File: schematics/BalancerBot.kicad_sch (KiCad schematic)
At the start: 7 parts, among them M1 Motor_DC, M2 Motor_DC, U1 MCP73871, U2 L298N

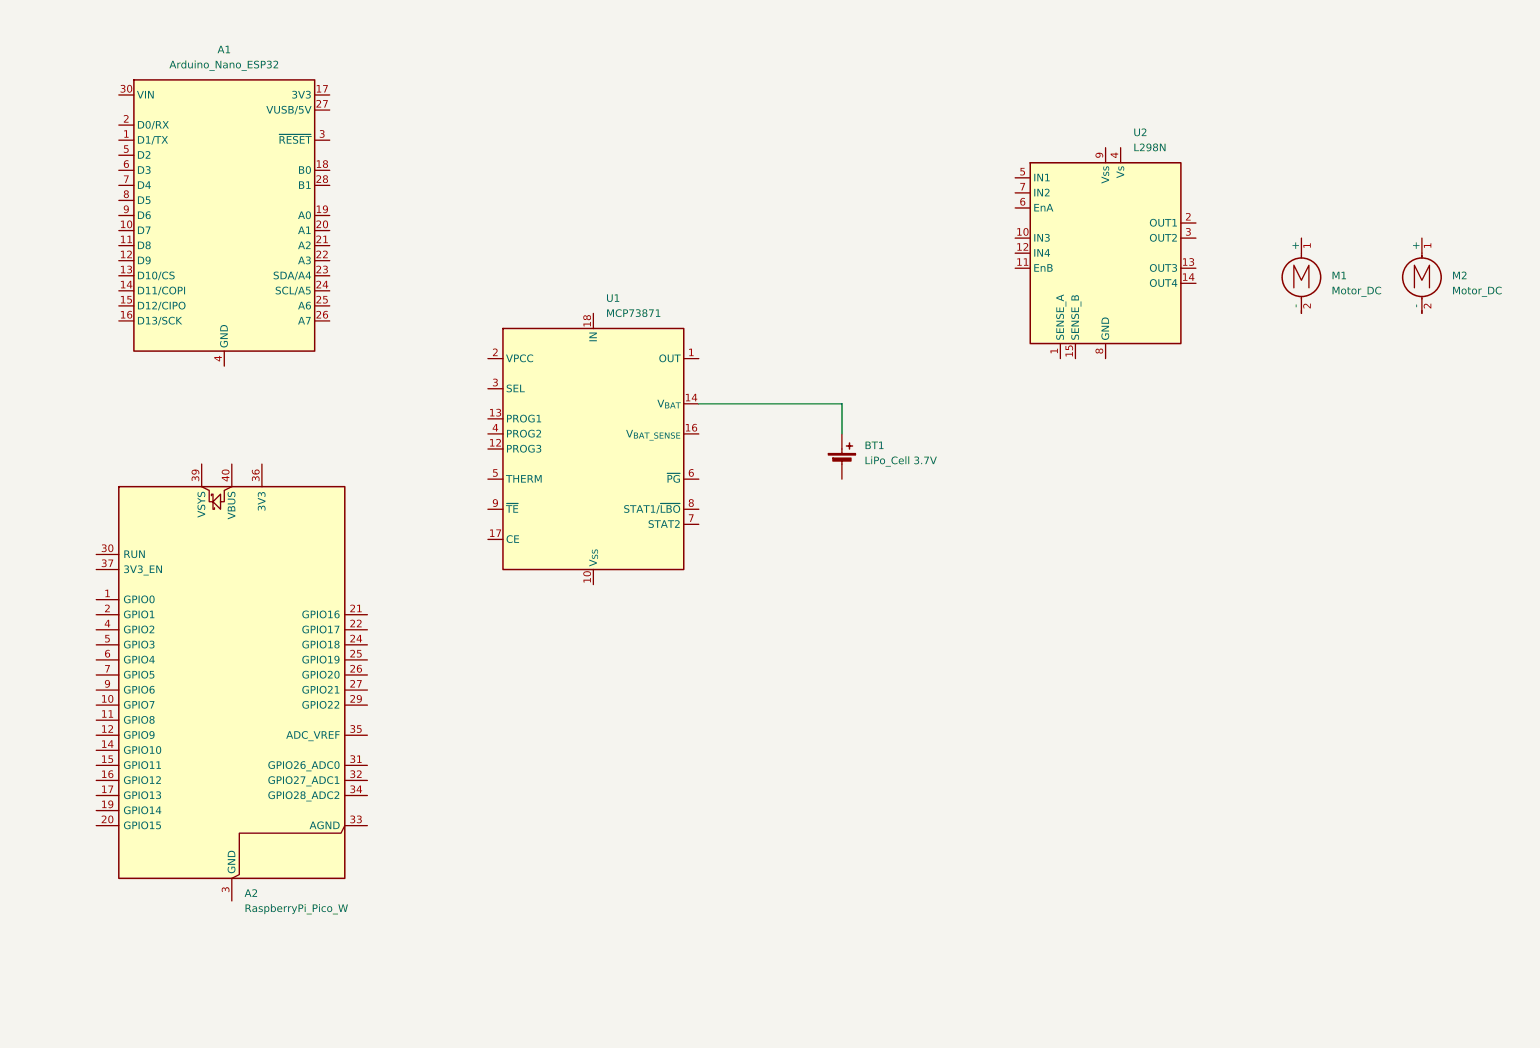
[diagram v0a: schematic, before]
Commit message: Update
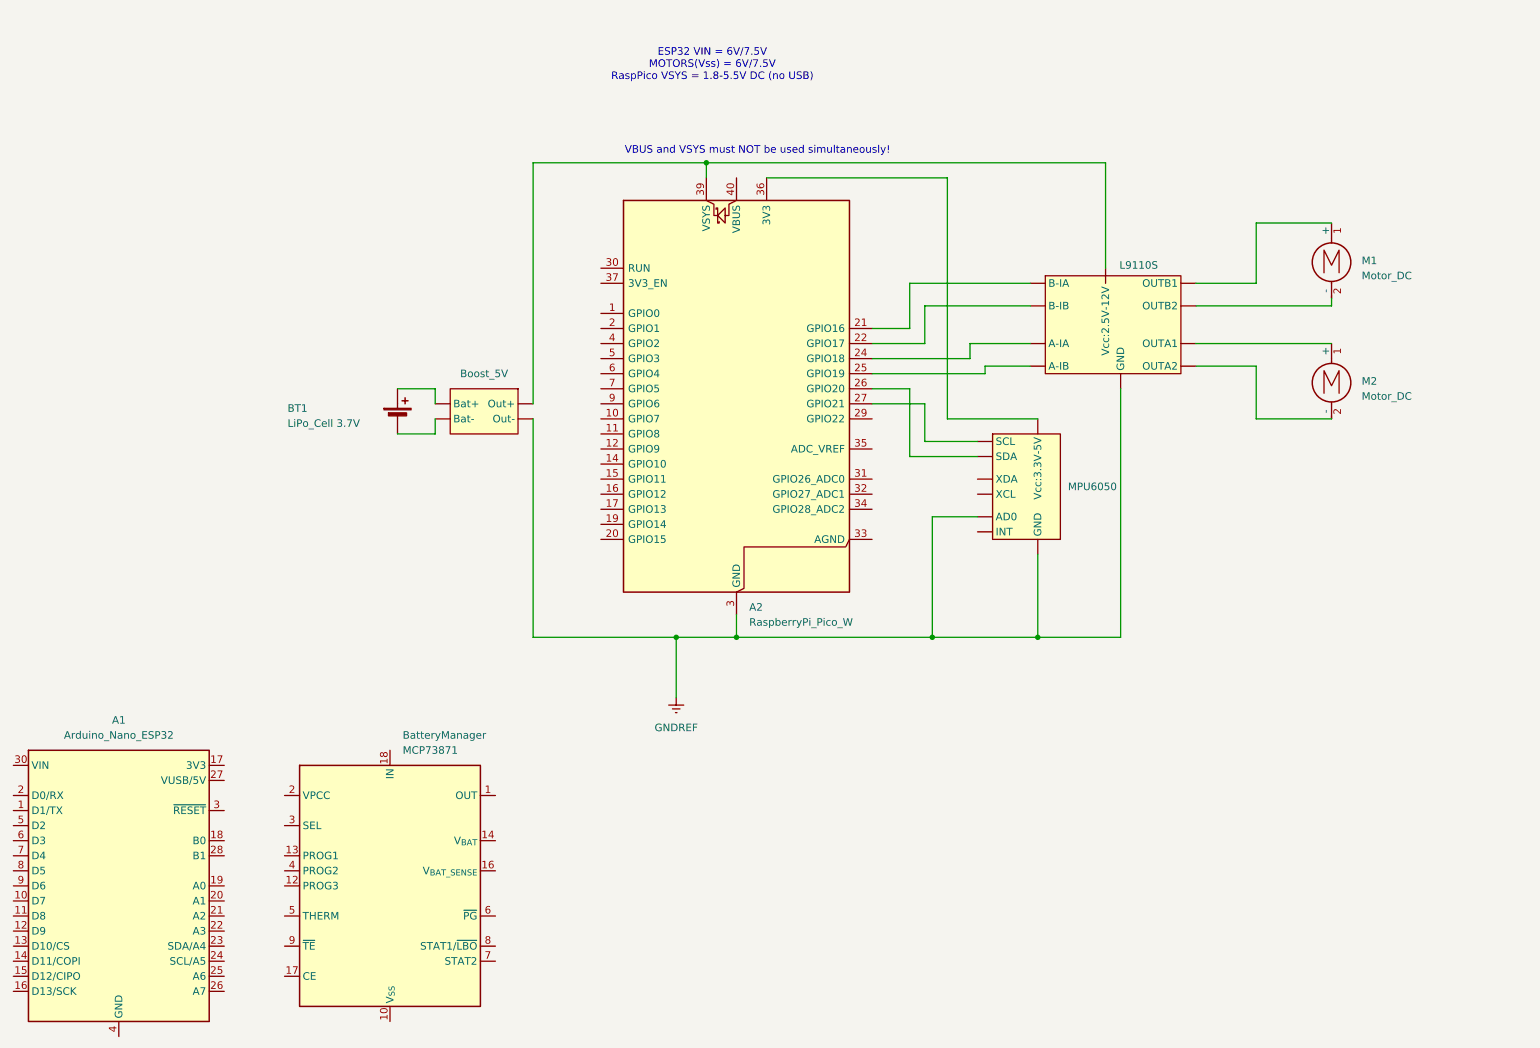
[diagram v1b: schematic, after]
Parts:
- removed U2: L298N, Package_TO_SOT_THT:TO-220-15_P2.54x5.08mm_StaggerOdd_Lead4.58mm_Vertical, symbol Driver_Motor:L298N
- added Boost_5V: (no value), symbol 1MyLibrary:Power_Boost_module_-_5V_0.5A_JST
- added L9110S: (no value), symbol MyLibrary:L9110S
- added MPU6050: (no value), symbol 1MyLibrary:SEN-MPU6050
- renumbered U1 to BatteryManager
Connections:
- net at M2.1 (+): now also L9110S. (OUTA2)
- net at M2.2 (-): now also L9110S. (OUTA2)
- net at BatteryManager.14 (V_{BAT}), BatteryManager.15 (V_{BAT}): no longer BT1.1 (+)
- net at BT1.2 (-): now also Boost_5V. (Bat-)
- net at M1.1 (+): now also L9110S. (OUTA2)
- net at M1.2 (-): now also L9110S. (OUTA2)
- net GNDREF: now reaches A2.13 (GND), A2.18 (GND), A2.23 (GND), A2.28 (GND), A2.3 (GND), A2.38 (GND), A2.8 (GND)
- net GNDREF: now also Boost_5V. (Bat-), L9110S. (OUTA2), MPU6050. (GND)
- net at A2.21 (GPIO16): now also L9110S. (OUTA2)
- net at A2.22 (GPIO17): now also L9110S. (OUTA2)
- net at A2.24 (GPIO18): now also L9110S. (OUTA2)
- net at A2.25 (GPIO19): now also L9110S. (OUTA2)
- net at A2.26 (GPIO20): now also MPU6050. (GND)
- net at A2.27 (GPIO21): now also MPU6050. (GND)
- net at A2.36 (3V3): now also MPU6050. (GND)
- net at A2.39 (VSYS): now also Boost_5V. (Bat-), L9110S. (OUTA2)
- new net: BT1.1 (+), Boost_5V. (Bat-)
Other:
- note added: "ESP32 VIN = 6V/7.5V MOTORS(Vss) = 6V/7.5V RaspPico VSYS = 1.8-5.5V DC (no USB)"
- note added: "VBUS and VSYS must NOT be used simultaneously!"
- moved on the sheet: A1, A2, BT1, BatteryManager, M1, M2

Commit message: Update schematic
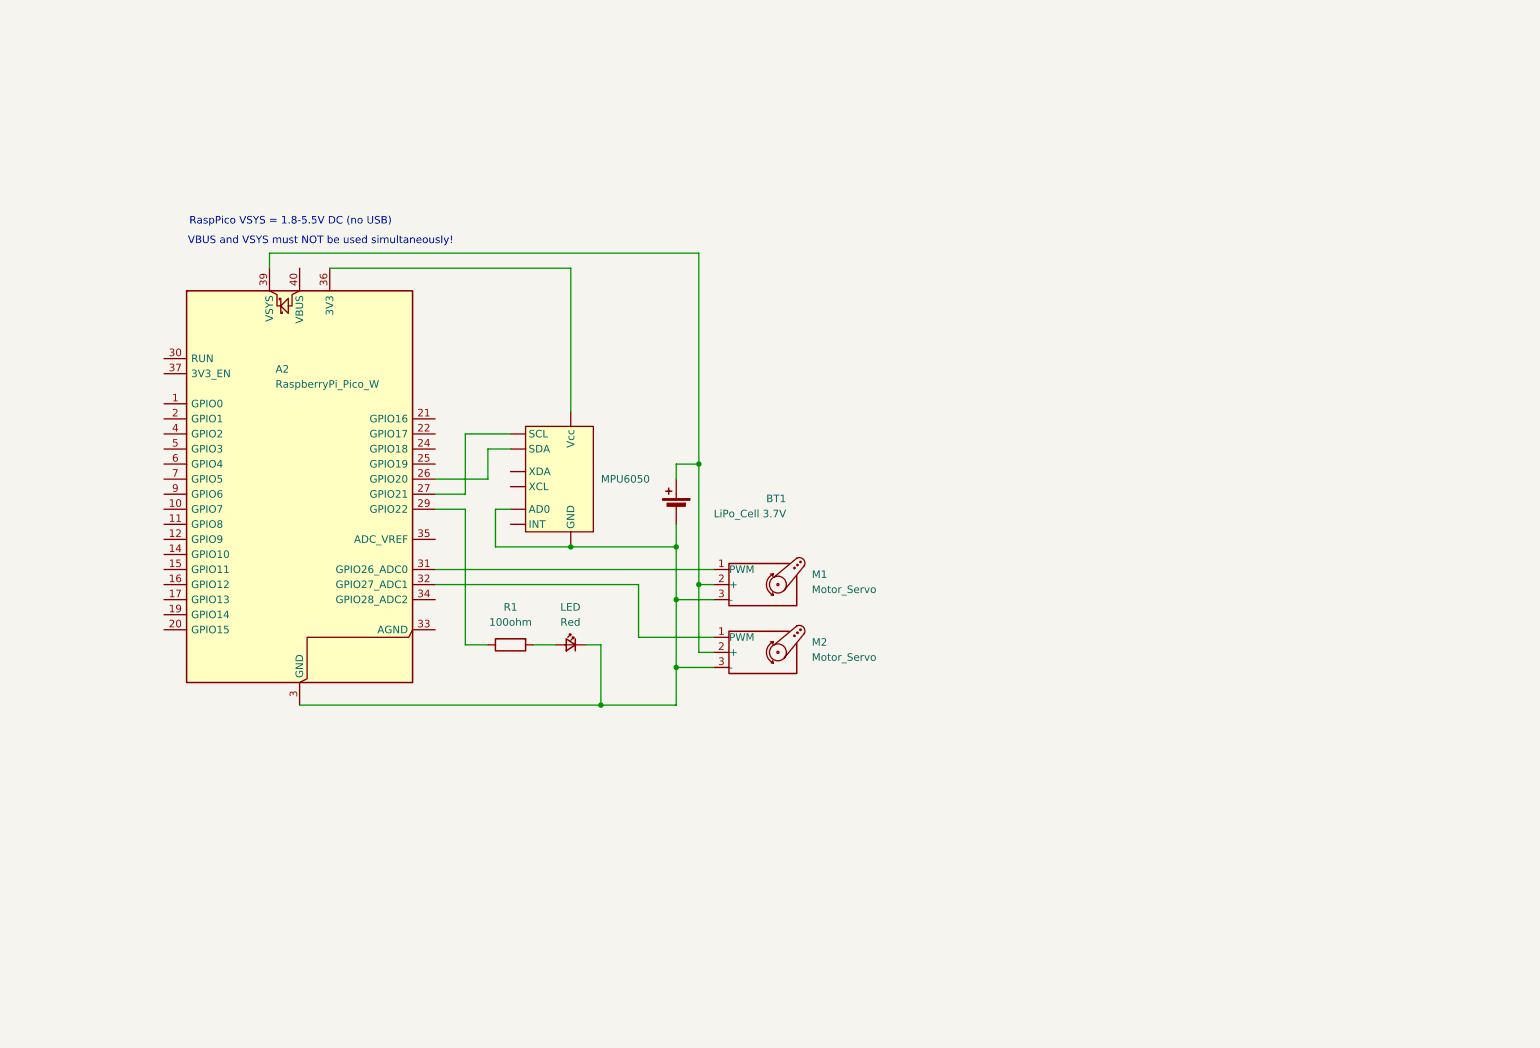
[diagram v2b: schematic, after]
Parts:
- removed A1: Arduino_Nano_ESP32, Module:Arduino_Nano, symbol MCU_Module:Arduino_Nano_ESP32
- removed BatteryManager: MCP73871, Package_DFN_QFN:QFN-20-1EP_4x4mm_P0.5mm_EP2.5x2.5mm, symbol Battery_Management:MCP73871
- removed Boost_5V: (no value), symbol 1MyLibrary:Power_Boost_module_-_5V_0.5A_JST
- removed L9110S: (no value), symbol MyLibrary:L9110S
- removed M1, M2: Motor_DC, symbol Motor:Motor_DC
- added LED: Red, PCM_SparkFun-LED:LED_0402_1005Metric_Red, symbol PCM_SparkFun-LED:LED_Red_0402
- added M1, M2: Motor_Servo, symbol Motor:Motor_Servo
- added R1: 100ohm, symbol PCM_Resistor_AKL:R_Generic
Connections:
- net at MPU6050. (GND): now also A2.36 (3V3)
- net at BT1.1 (+): now also A2.39 (VSYS), M1.2 (+), M2.2 (+)
- net at BT1.2 (-): now also A2.13 (GND), A2.18 (GND), A2.23 (GND), A2.28 (GND), A2.3 (GND), A2.38 (GND), A2.8 (GND), MPU6050. (GND), LED.1 (K), M1.3 (-), M2.3 (-)
- net at A2.29 (GPIO22): now also R1.2
- net at A2.31 (GPIO26_ADC0): now also M1.1 (PWM)
- net at A2.32 (GPIO27_ADC1): now also M2.1 (PWM)
- removed net GNDREF: A2.13 (GND), A2.18 (GND), A2.23 (GND), A2.28 (GND), A2.3 (GND), A2.38 (GND), A2.8 (GND), MPU6050. (GND)
- new net: LED.2 (A), R1.1
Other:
- note added: "RaspPico VSYS = 1.8-5.5V DC (no USB)"
- note removed: "ESP32 VIN = 6V/7.5V MOTORS(Vss) = 6V/7.5V RaspPico VSYS = 1.8-5.5V DC (no USB)"
- moved on the sheet: A2, BT1, MPU6050

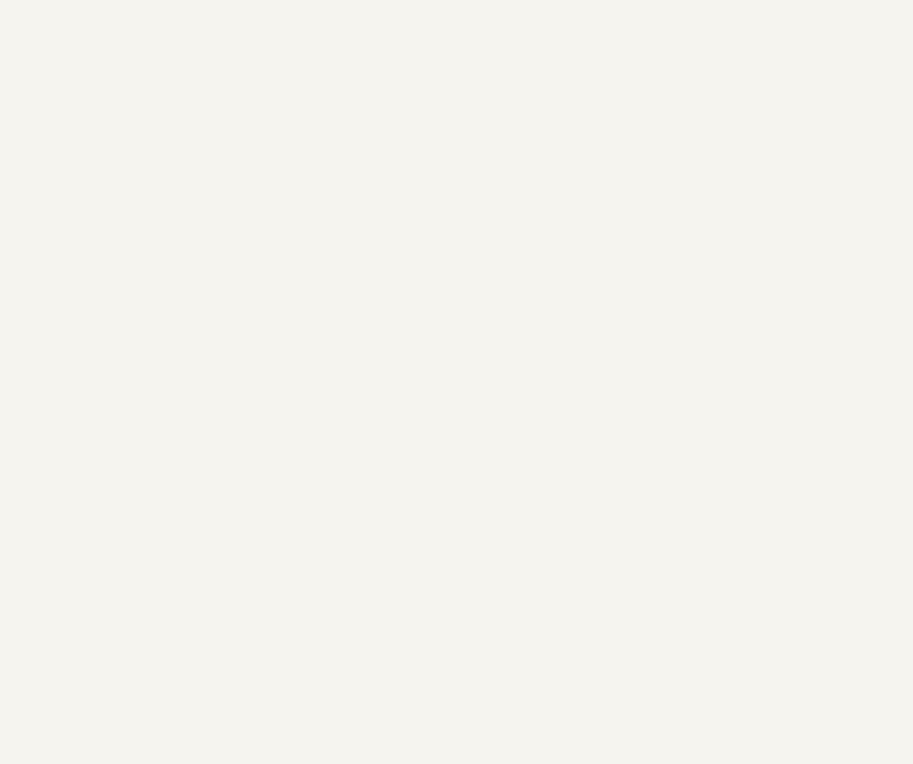
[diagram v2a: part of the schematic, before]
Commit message: 9dof IMU testing
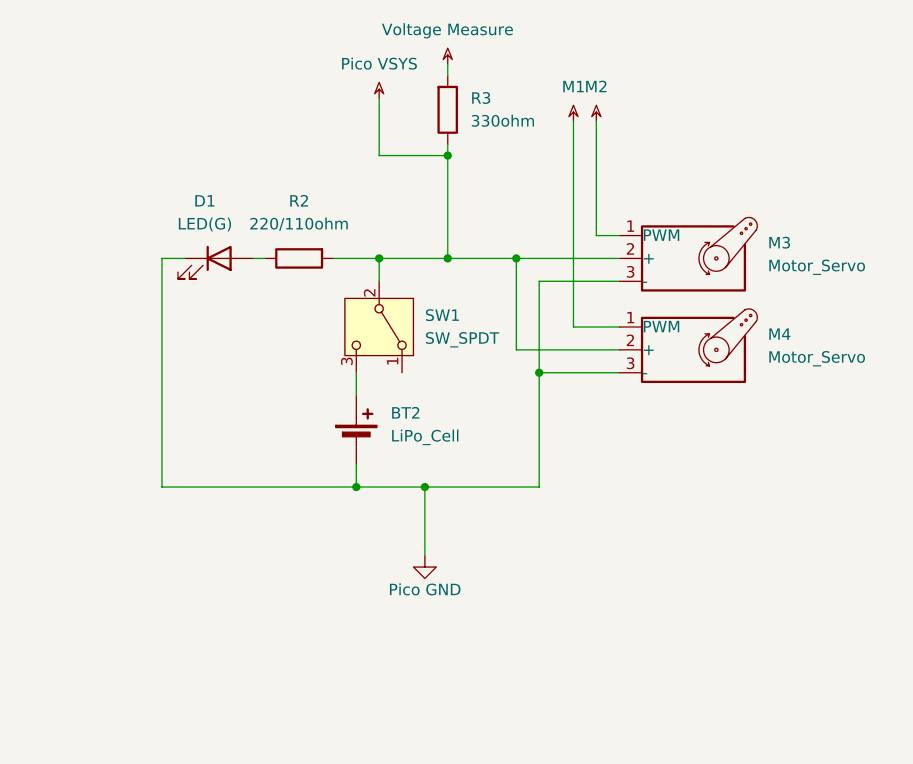
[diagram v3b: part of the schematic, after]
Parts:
- added BT2: LiPo_Cell, symbol Device:Battery_Cell
- added D1: LED(G), symbol Device:LED
- added M3, M4: Motor_Servo, symbol Motor:Motor_Servo
- added R2: 220/110ohm, symbol PCM_Resistor_AKL:R_Generic
- added R3: 330ohm, symbol PCM_Resistor_AKL:R_Generic
- added SW1: SW_SPDT, symbol Switch:SW_SPDT
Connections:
- net at MPU6050. (GND): now also A2.36 (3V3)
- new net: BT2.1 (+), SW1.3 (C)
- new net: D1.2 (A), R2.2
- new net M1: M4.1 (PWM)
- new net M2: M3.1 (PWM)
- new net Pico GND: BT2.2 (-), D1.1 (K), M3.3 (-), M4.3 (-)
- new net Pico VSYS: M3.2 (+), M4.2 (+), R2.1, R3.2, SW1.2 (B)
- new net Voltage Measure: R3.1
